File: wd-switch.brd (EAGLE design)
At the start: 40.3 x 59.7 mm, 16 parts, among them Q1 BC337, Q2 IRF530, Q3 IRF530, X1 KUSBVX

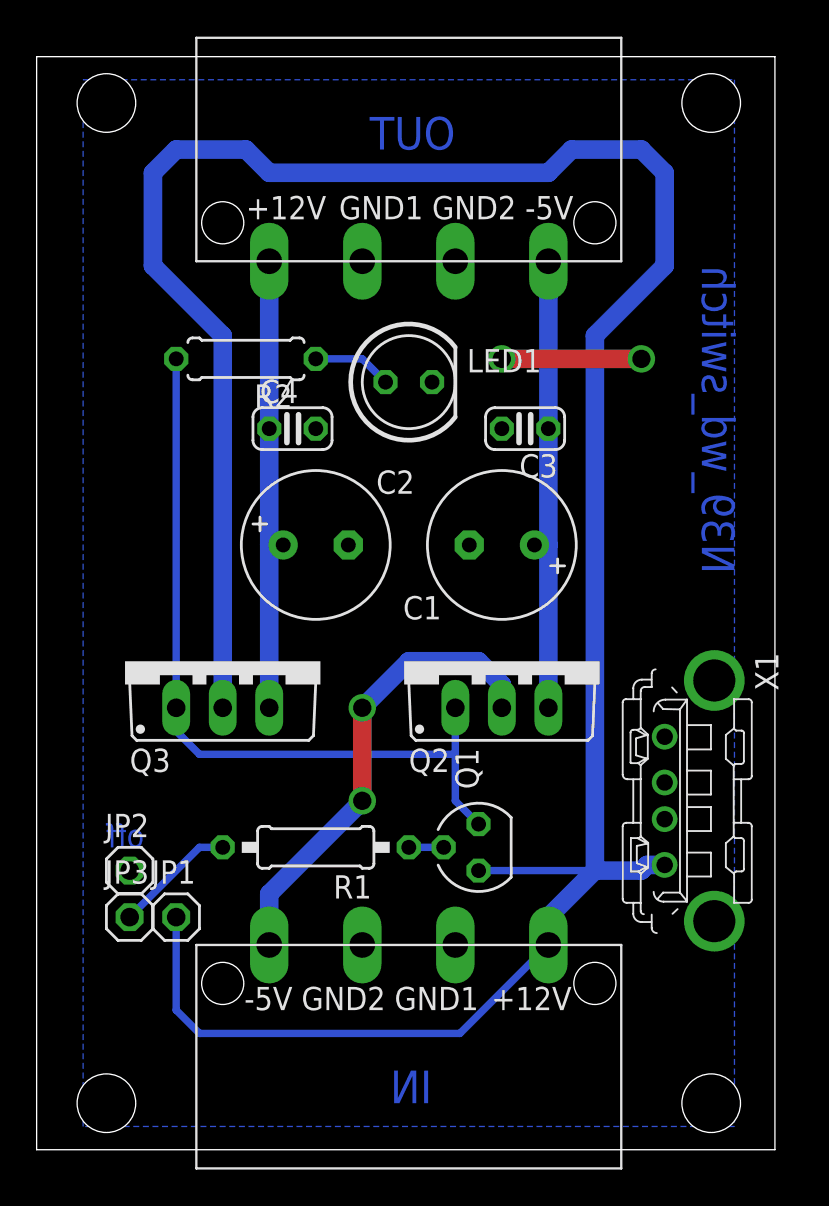
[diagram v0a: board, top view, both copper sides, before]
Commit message: Korrigiertes Design
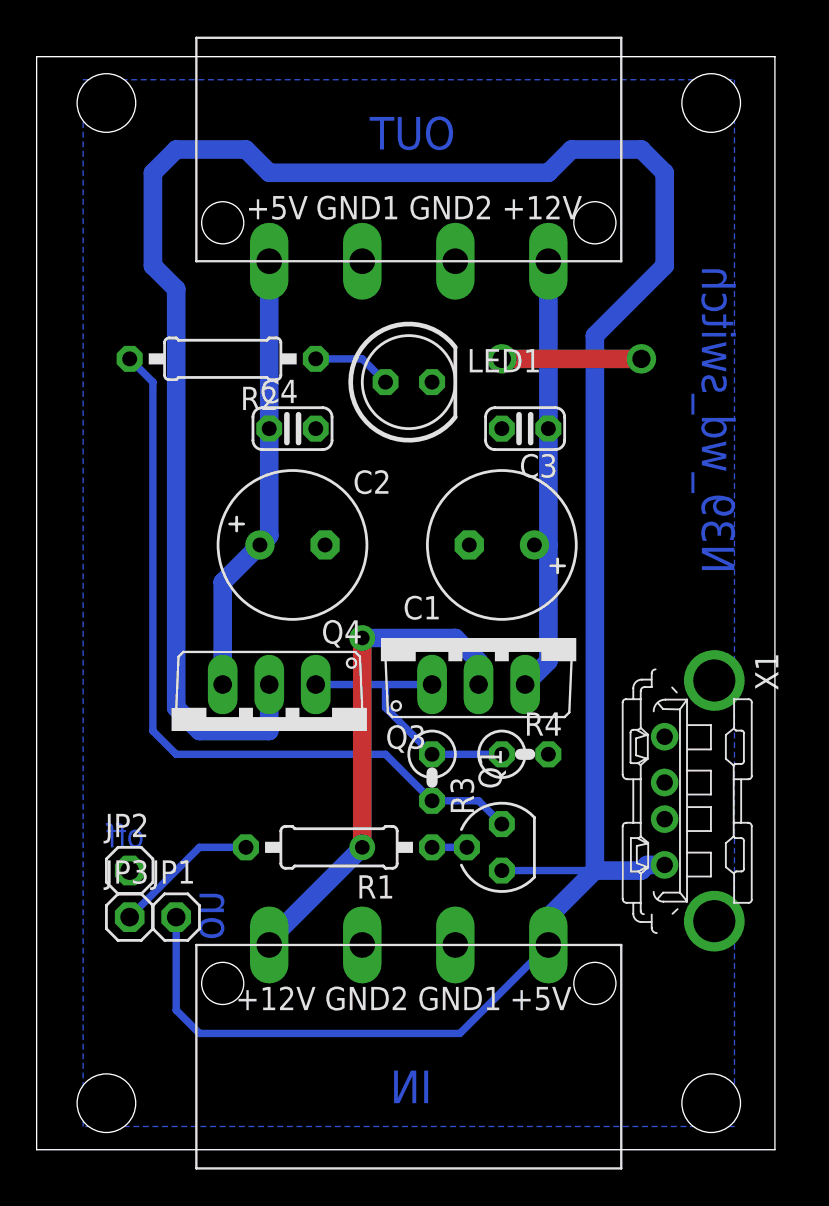
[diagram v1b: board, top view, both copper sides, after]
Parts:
- removed Q2: IRF530, transistor-power:TO220BV
- added Q4: IRL540N, n39:TO220V
- added R3: 100R, resistor:0207/2V
- added R4: 100K, resistor:0207/2V
- Q3: value IRF530 -> IRL540N; device transistor-power:TO220BV -> n39:TO220V
- R1: value 330R -> 150R
- R2: device resistor:0207/7 -> resistor:0207/10
- moved Q3 14.0 mm to (24.1, 27.9)
- moved R1 1.27 mm to (16.5, 16.5)
- moved C2 1.27 mm to (14.0, 33.0)
- moved Q1 1.27 mm to (25.4, 16.5)
- moved R2 1.27 mm to (10.2, 43.2)
- renumbered U$1 to IN, U$2 to OUT
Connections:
- new net N$11: Q1.E, R2.2, R3.2
- net GND: now also R4.2
- net N$1: now also Q3.1, Q4.1, R3.1, R4.1; no longer Q1.E, Q2.G, Q3.G, R2.2
- net N$2: now also Q3.3; no longer Q2.S
- net N$4: now also OUT.+5V, Q4.3; no longer OUT.-5V, Q3.S
- net VCC: now also IN.+5V, Q4.2; no longer IN.-5V, Q3.D
- net VDD: now also Q3.2; no longer Q2.D
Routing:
- net N$11: track 0.00 -> 42.0 mm
- net N$1: track 43.0 -> 15.0 mm
- net VCC: track 143.8 -> 149.7 mm
- net VDD: track 25.3 -> 27.0 mm
- net N$5: track 6.66 -> 7.93 mm
- net N$4: track 25.1 -> 24.2 mm
- net N$2: track 25.1 -> 24.4 mm
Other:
- board text added: "on"
